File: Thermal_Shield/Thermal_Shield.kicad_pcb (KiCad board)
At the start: 2 copper layers, 19 parts, among them J1 Screw_Terminal_01x03, J2 Barrel_Jack_Switch, Q1 BC337, Q2 BC337, Q3 BC337, U1 LM35-D, U2 LM311

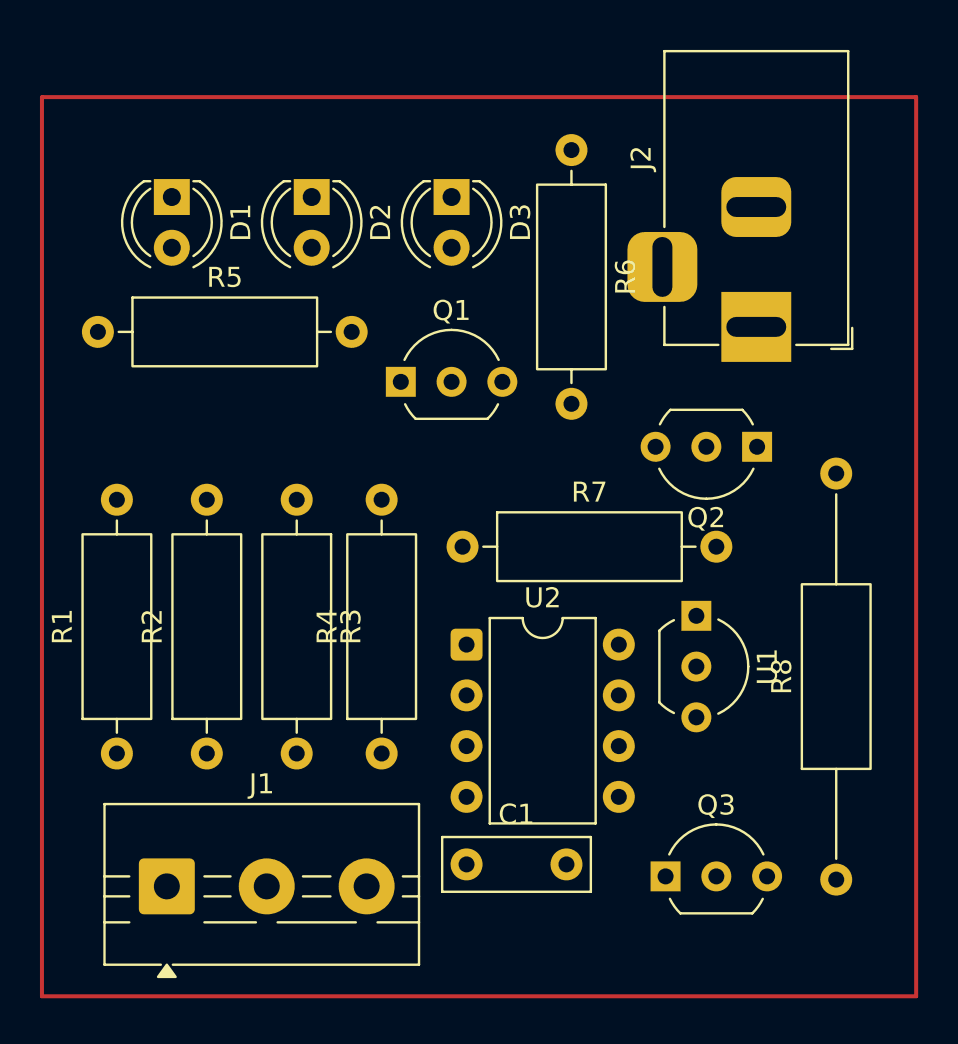
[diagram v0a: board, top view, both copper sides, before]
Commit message: Connections
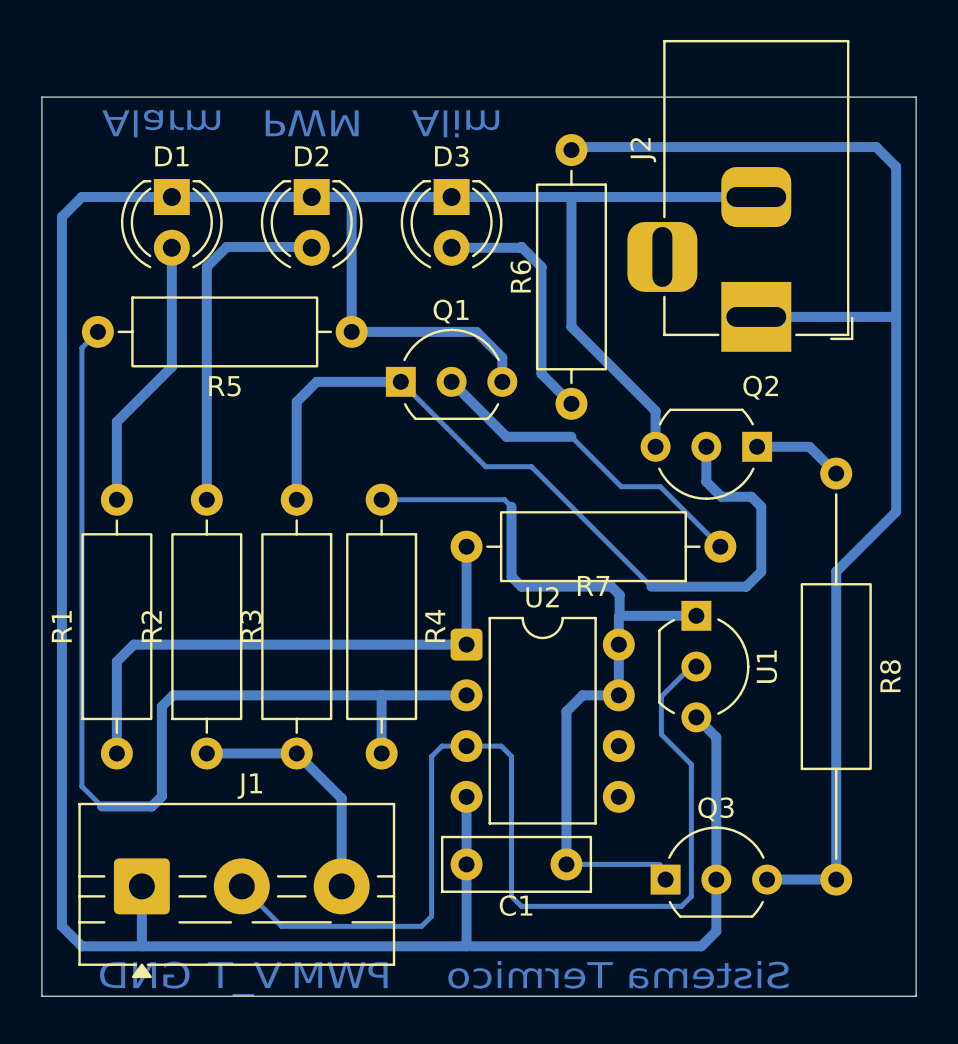
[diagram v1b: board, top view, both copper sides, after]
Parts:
- U1: value LM35-D -> LM35-LP
- moved R7 19.9 mm to (58.0, 57.5), turned to 180 degrees
- moved C1 5.00 mm to (50.2, 73.4), turned to 180 degrees
- moved R4 4.68 mm to (41.0, 55.1), turned to -90 degrees
- moved J1 1.25 mm to (29.0, 74.5)
- moved J2 0.50 mm to (59.8, 46.0)
- moved Q3 0.16 mm to (55.2, 74.2)
- renumbered R7 to R4, R4 to R7
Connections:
- C1 pad 2: Net-(U2-GND) -> GND
- J1 pad 1: PMW -> GND
- J1 pad 3: GND -> PWM
- Q1 pad 1: GND -> Net-(Q1-C)
- Q1 pad 3: Net-(Q1-E) -> GND
- Q2 pad 2: Net-(Q1-E) -> Net-(Q1-C)
- R3 pad 1: Net-(Q1-E) -> Net-(Q1-C)
- R4 pad 1: Net-(U1-+V_{S}) -> Net-(Q3-C)
- U1 pad 1: V_T -> Net-(Q3-C)
- U1 pad 2: unconnected-(U1-NC-Pad2) -> V_T
- U1 pad 3: unconnected-(U1-NC-Pad3) -> GND
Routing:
- net GND: track 0.00 -> 156.0 mm
- net IN_12: track 0.00 -> 64.2 mm
- net V_T: track 0.00 -> 52.4 mm
- net Net-(U2-+): track 0.00 -> 50.6 mm
- net Net-(Q1-C): track 0.00 -> 41.4 mm
- net Net-(Q3-C): track 0.00 -> 41.2 mm
- net Net-(U2-GND): track 0.00 -> 27.4 mm
- net Net-(D2-A): track 0.00 -> 17.4 mm
- net Net-(Q1-B): track 0.00 -> 16.9 mm
- net Net-(D1-A): track 0.00 -> 13.7 mm
- net PWM: track 0.00 -> 12.8 mm
- net Net-(D3-A): track 0.00 -> 12.6 mm
- net Net-(Q2-C): track 0.00 -> 4.52 mm
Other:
- board outline added: 43.8 x 45 mm
- board text added: "Alarm"
- board text added: "Alim"
- board text added: "GND"
- board text added: "PWM"
- board text added: "Sistema Termico"
- board text added: "V_T"
